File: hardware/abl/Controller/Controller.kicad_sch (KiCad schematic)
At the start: 27 parts, among them IC1 LSF0204PWJ, IC2 FXL6408UMX, IC3 VEML6040A3OG, IC4 FXL6408UMX, J1 SFW20S-2STE1LF, J2 Conn_02x03_Odd_Even, J3 Conn_02x03_Odd_Even, J4 PRT-14417, J5 Conn_02x04_Odd_Even, Q2 AO3401A, Q4 AO3401A, U1 INA219AxD

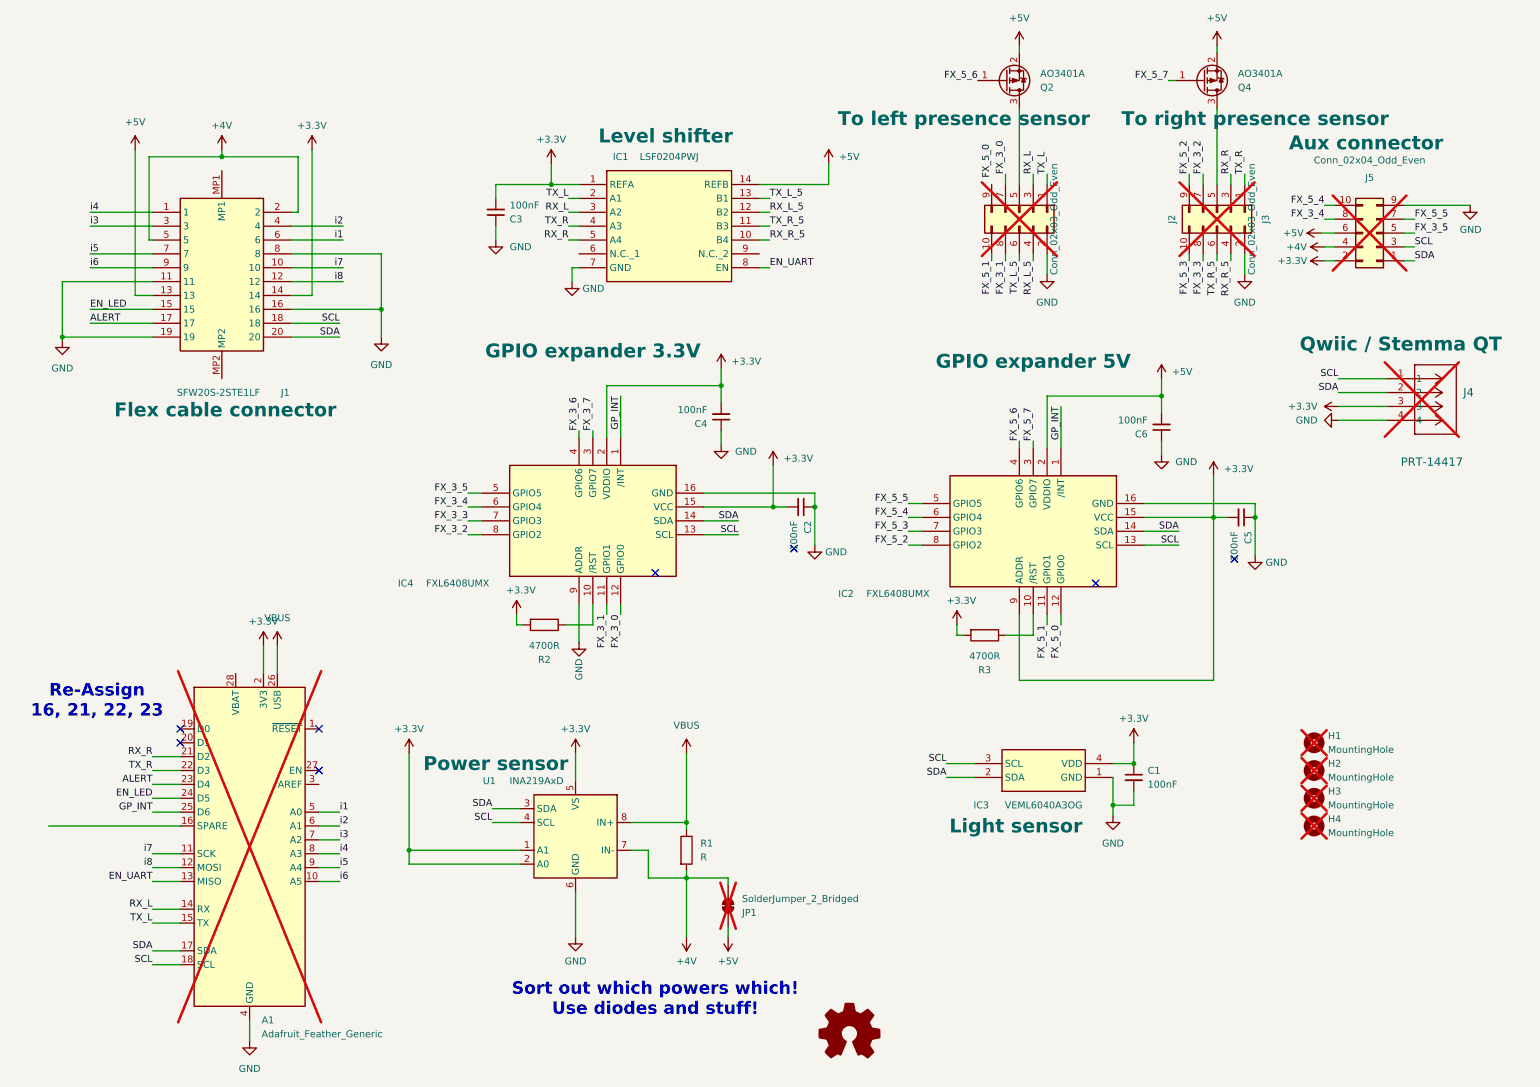
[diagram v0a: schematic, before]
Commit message: Metadata and minor cleanup, documentation and typo fix.
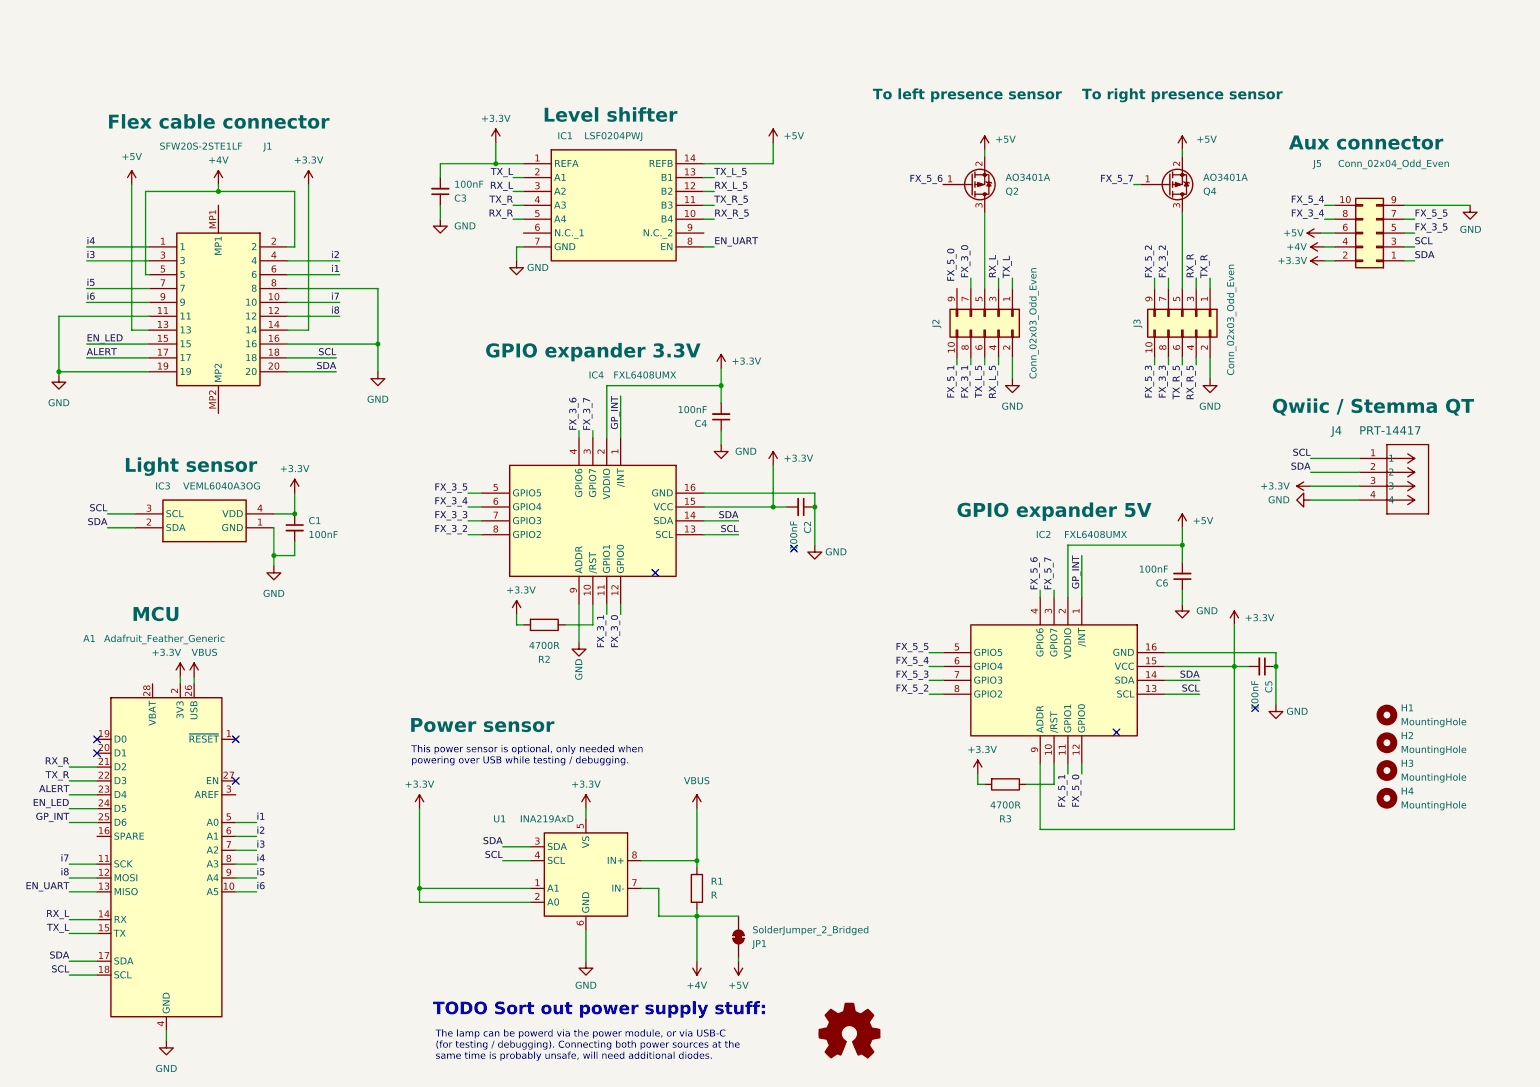
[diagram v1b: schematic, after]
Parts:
- A1: now fitted; now left out of the parts list
- H1, H2, H3, H4, J2, J3, J4, J5, JP1: now fitted
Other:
- note added: "TODO Sort out power supply stuff:"
- note removed: "Re-Assign 16, 21, 22, 23"
- note removed: "Sort out which powers which! Use diodes and stuff!"
- title: (none) -> besteLampe! ABL Controller Module
- moved on the sheet: C1, C3, C5, C6, IC1, IC2, IC3, J1, Q2, Q4, R1, R3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
